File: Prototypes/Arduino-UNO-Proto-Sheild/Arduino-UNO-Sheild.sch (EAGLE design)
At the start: 1 part, among them J1 ARDUINO_R3_SHIELD

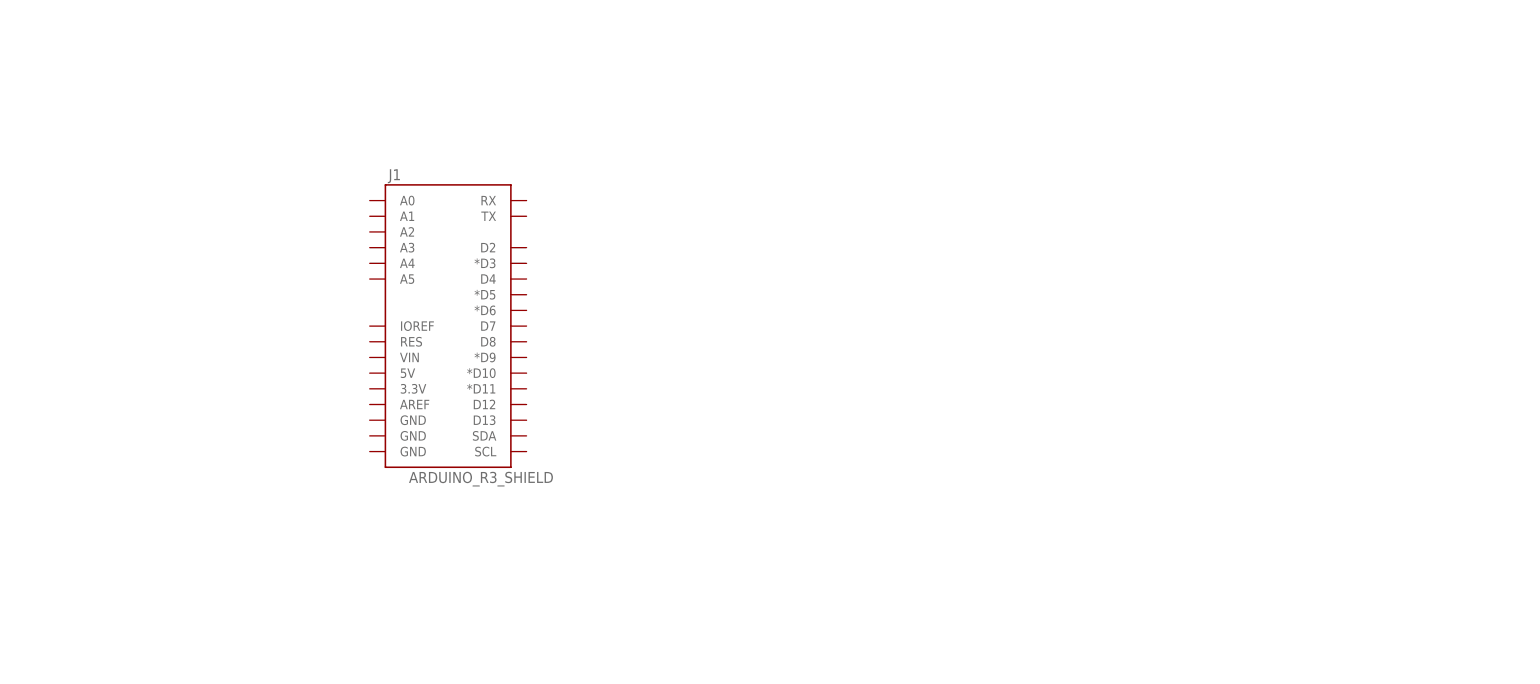
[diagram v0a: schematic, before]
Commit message: Fixes
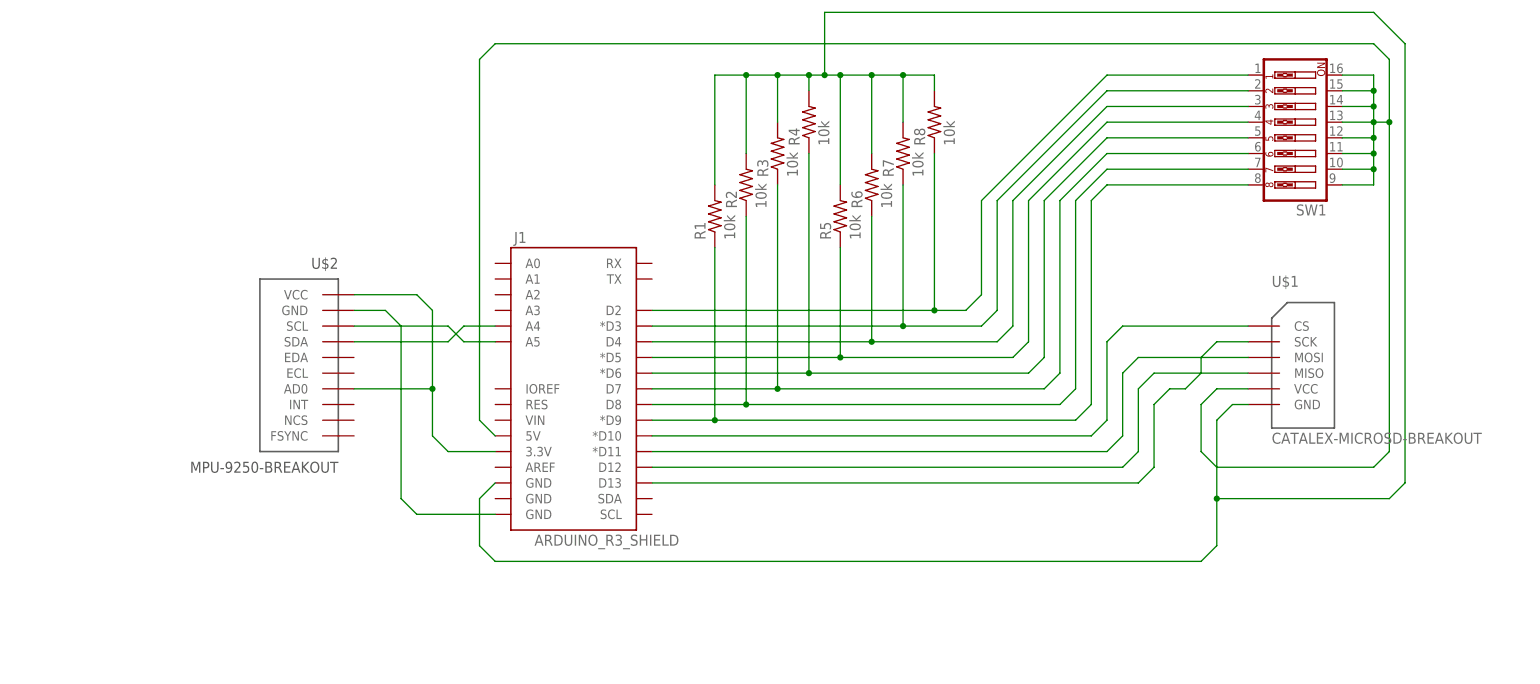
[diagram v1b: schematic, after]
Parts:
- added R1, R2, R3, R4, R5, R6, R7, R8: 10k, SparkFun-Passives:RESISTORKIT
- added SW1: (no value), SparkFun-Electromechanical:SW_DIP-8
- added U$1: CATALEX-MICROSD-BREAKOUT, Modules:CATALEX-MICROSD-BREAKOUT
- added U$2: MPU-9250-BREAKOUT, Modules:MPU-9250-BREAKOUT
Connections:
- new net N$1: J1.A4, U$2.SDA
- new net N$10: J1.*D9, R1.1, SW1.8
- new net N$11: J1.D8, R2.1, SW1.7
- new net N$12: J1.D7, R3.1, SW1.6
- new net N$13: J1.*D6, R4.1, SW1.5
- new net N$14: J1.*D5, R5.1, SW1.4
- new net N$15: J1.D4, R6.1, SW1.3
- new net N$16: J1.*D3, R7.1, SW1.2
- new net N$17: J1.D2, R8.1, SW1.1
- new net N$18: J1.5V, SW1.10, SW1.11, SW1.12, SW1.13, SW1.14, SW1.15, SW1.16, SW1.9, U$1.VCC
- new net N$2: J1.A5, U$2.SCL
- new net N$20: J1.GND@2, R1.2, R2.2, R3.2, R4.2, R5.2, R6.2, R7.2, R8.2, U$1.GND
- new net N$3: J1.3.3V, U$2.AD0, U$2.VCC
- new net N$4: J1.GND@0, U$2.GND
- new net N$6: J1.*D10, U$1.CS
- new net N$7: J1.D13, U$1.SCK
- new net N$8: J1.*D11, U$1.MOSI
- new net N$9: J1.D12, U$1.MISO
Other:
- moved on the sheet: J1

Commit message: Fixes
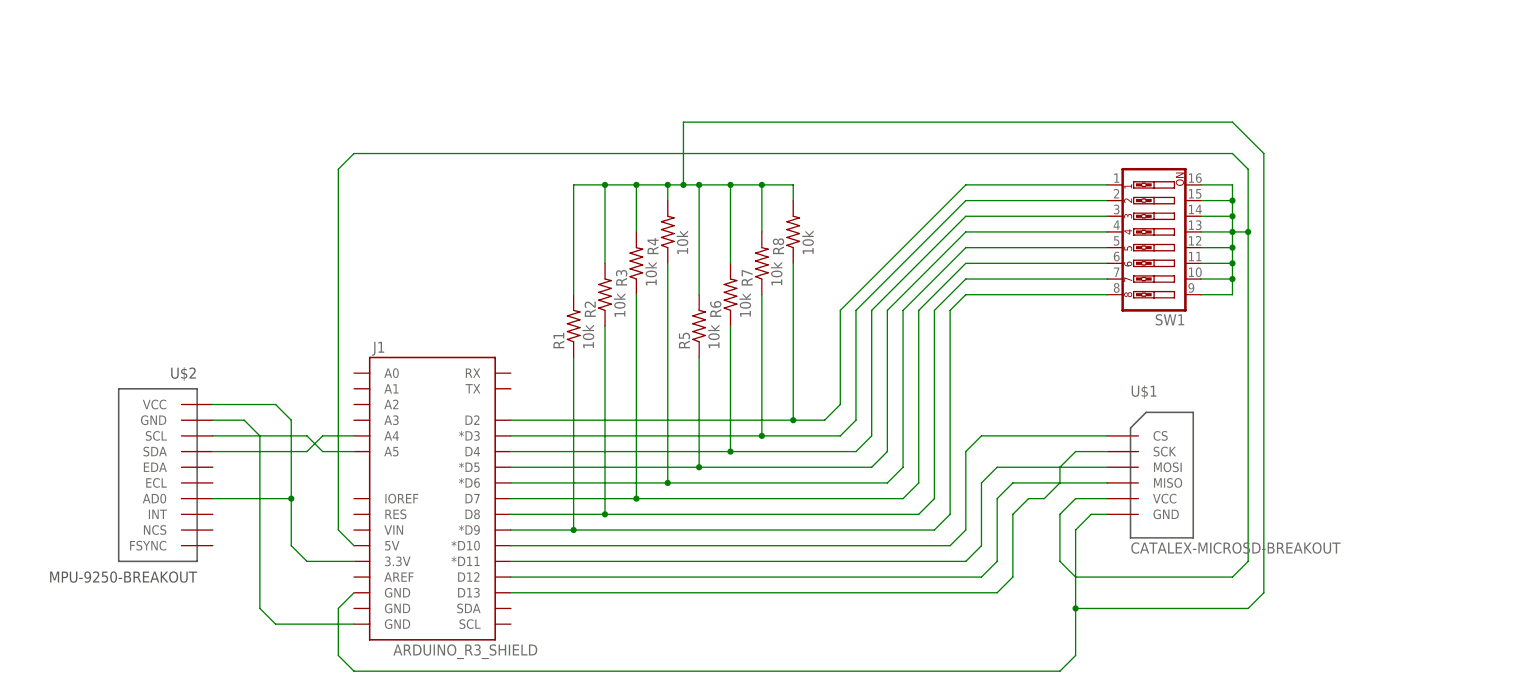
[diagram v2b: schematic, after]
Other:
- moved on the sheet: J1, R1, R2, R3, R4, R5, R6, R7, R8, SW1, U$1, U$2
